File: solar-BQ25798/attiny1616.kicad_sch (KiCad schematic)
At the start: 26 parts, among them J1901 TC2030, Q1901 2N7002, U1 HDC2080, U106 M24C02-WMN, U1902 ATtiny1616-M

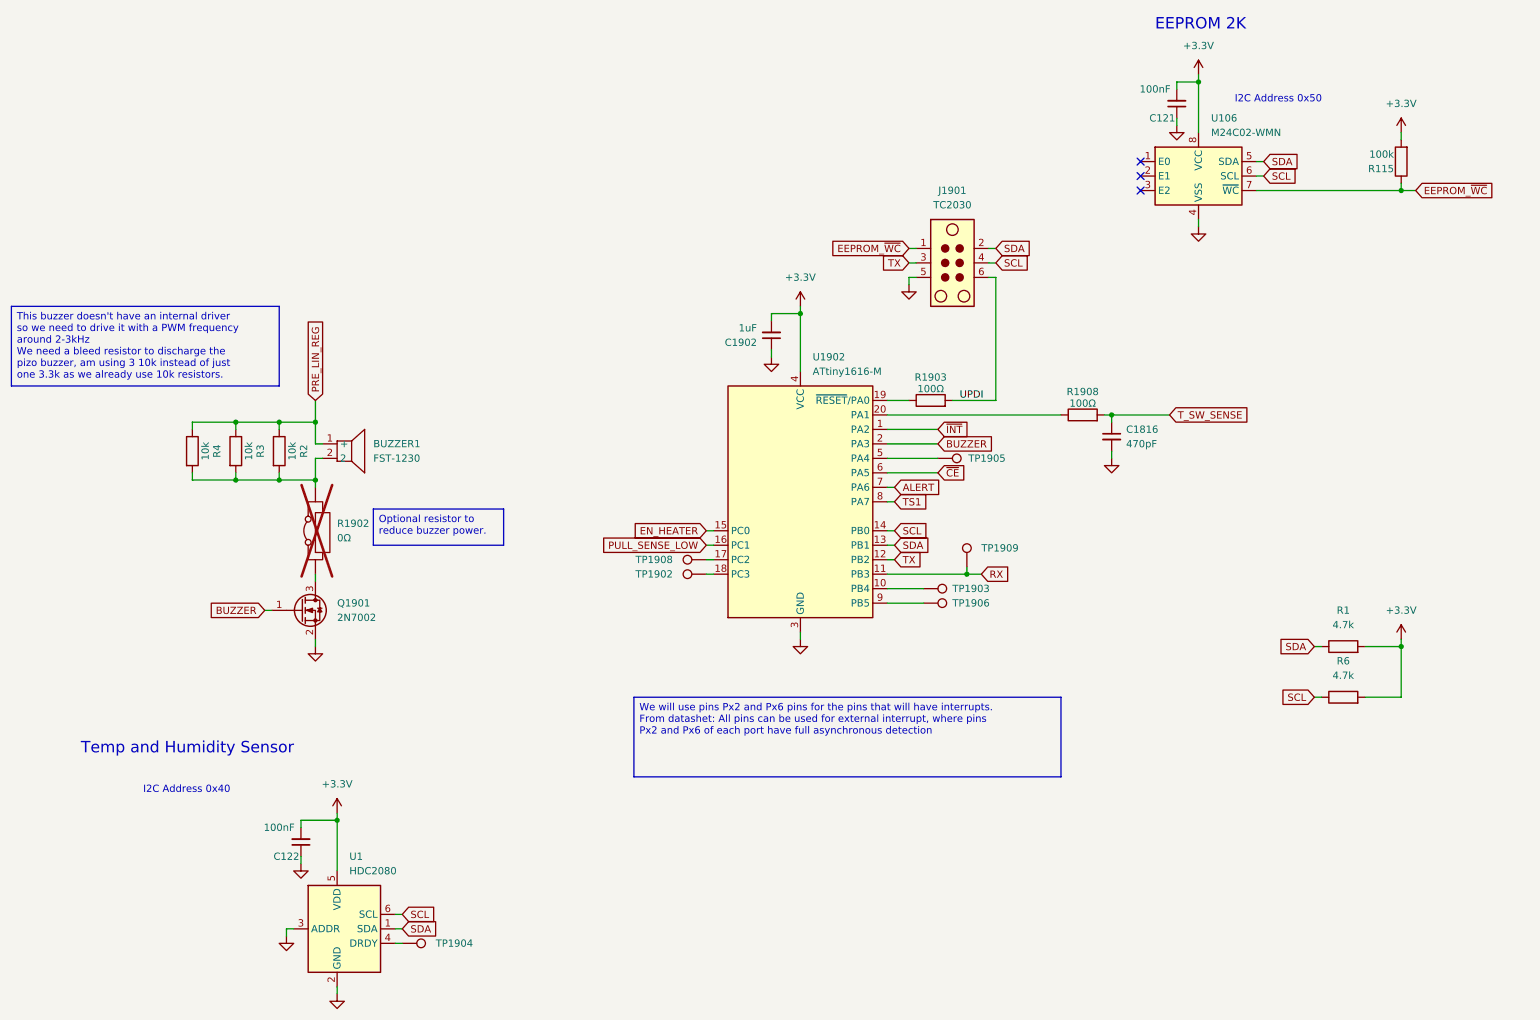
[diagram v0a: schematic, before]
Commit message: Tidy up
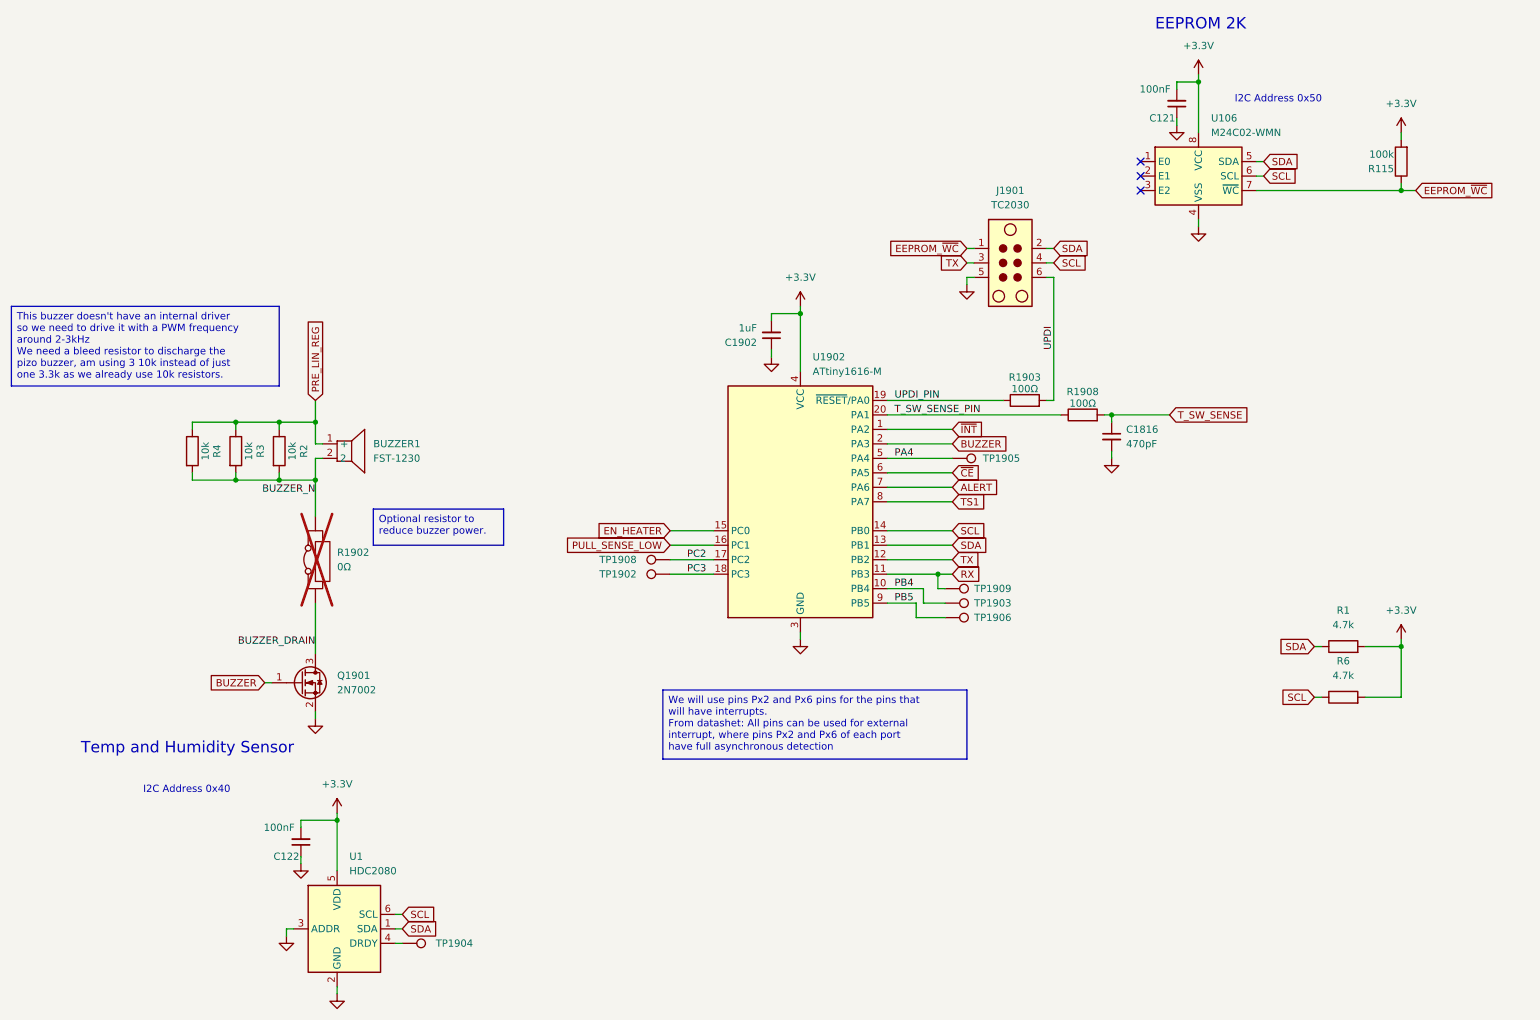
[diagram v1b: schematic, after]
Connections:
- net BUZZER_DRAIN: now reaches Q1901.3 (D), R1902.1 (A)
- net BUZZER_N: now reaches BUZZER1.2, R1902.2 (B), R2.2, R3.2, R4.2
- net PB4: now reaches TP1903.1, U1902.10 (PB4)
- net T_SW_SENSE_PIN: now reaches R1908.1, U1902.20 (PA1)
- net UPDI_PIN: now reaches R1903.1, U1902.19 (~{RESET}/PA0)
- net PA4: now reaches TP1905.1, U1902.5 (PA4)
- net PC2: now reaches TP1908.1, U1902.17 (PC2)
- net PC3: now reaches TP1902.1, U1902.18 (PC3)
- net PB5: now reaches TP1906.1, U1902.9 (PB5)
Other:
- moved on the sheet: J1901, Q1901, R1902, R1903, TP1902, TP1903, TP1905, TP1906, TP1908, TP1909
